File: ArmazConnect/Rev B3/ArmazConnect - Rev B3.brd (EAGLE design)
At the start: 165 x 74 mm, 59 parts, among them X0 NC3FAV2, X1 NC3FAV2, X2 NC3FAV2, X3 NC3FAV2, X4 NC5FAV-SW, X5 NC5MAV-SW, X6 NC5FAV-SW, X8 87832-26

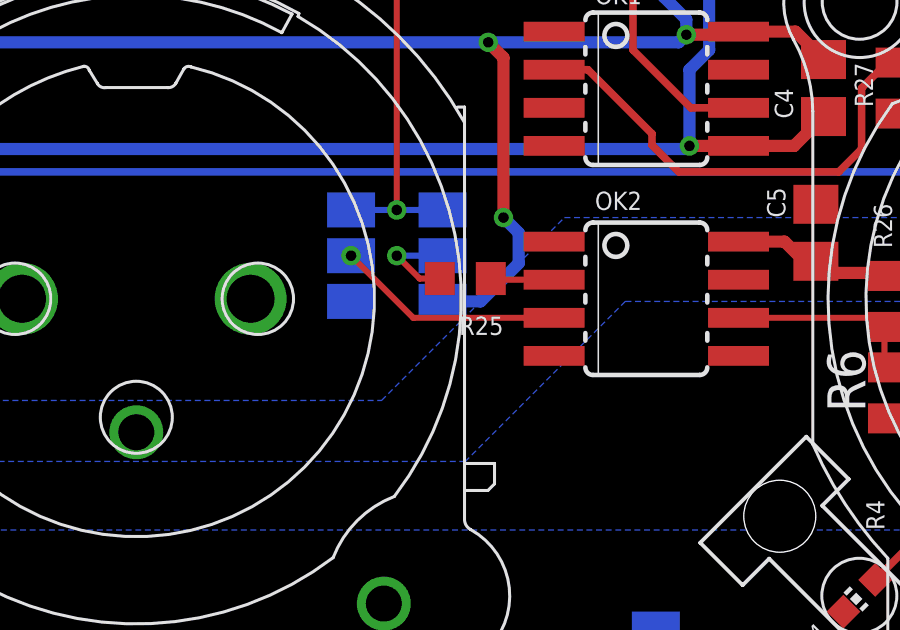
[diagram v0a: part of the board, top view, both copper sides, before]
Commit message: Revert "Update Armaz schematic and board, generate GERBER file"
This reverts commit 24852c679122bbaf0d2032972172e40d6d3f08fb.
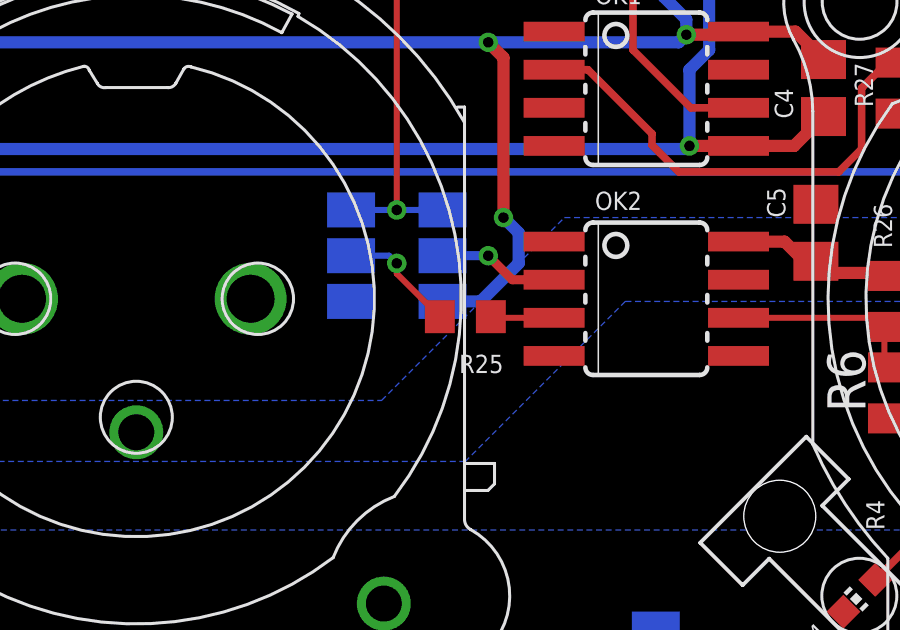
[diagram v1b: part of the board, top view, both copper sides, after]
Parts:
- moved R25 1.27 mm to (125.0, 57.4)
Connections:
- removed net N$10: OK2.2, R25.1
- removed net N$11: R25.2, SJ1.2
- new net N$17: OK2.3, R25.1
- new net UART5_TXD4: R25.2, SJ2.2
- net N$9: now also OK2.2, SJ1.2; no longer OK2.3, SJ2.2
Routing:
- net UART5_TXD4: track 0.00 -> 4.00 mm, vias 0 -> 1
- net N$9: track 7.63 -> 4.05 mm
- net N$11: track 3.28 -> 0.00 mm, vias 1 -> 0
- net N$17: track 0.00 -> 2.12 mm
- net N$10: track 2.12 -> 0.00 mm
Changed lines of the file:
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@@
 <layer number="14" name="Route14" color="1" fill="6" visible="no" active="no"/>
 <layer number="15" name="Route15" color="19" fill="6" visible="no" active="no"/>
-<layer number="16" name="Bottom" color="21" fill="1" visible="no" active="yes"/>
+<layer number="16" name="Bottom" color="21" fill="1" visible="yes" active="yes"/>
 <layer number="17" name="Pads" color="18" fill="1" visible="yes" active="yes"/>
 <layer number="18" name="Vias" color="38" fill="1" visible="yes" active="yes"/>
@@
 <layer number="20" name="Dimension" color="7" fill="1" visible="yes" active="yes"/>
 <layer number="21" name="tPlace" color="55" fill="1" visible="yes" active="yes"/>
-<layer number="22" name="bPlace" color="54" fill="1" visible="no" active="yes"/>
+<layer number="22" name="bPlace" color="54" fill="1" visible="yes" active="yes"/>
 <layer number="23" name="tOrigins" color="15" fill="1" visible="yes" active="yes"/>
-<layer number="24" name="bOrigins" color="15" fill="1" visible="no" active="yes"/>
-<layer number="25" name="tNames" color="55" fill="1" visible="yes" active="yes"/>
+<layer number="24" name="bOrigins" color="15" fill="1" visible="yes" active="yes"/>
+<layer number="25" name="tNames" color="55" fill="1" visible="no" active="yes"/>
 <layer number="26" name="bNames" color="54" fill="1" visible="no" active="yes"/>
-<layer number="27" name="tValues" color="53" fill="1" visible="yes" active="yes"/>
+<layer number="27" name="tValues" color="53" fill="1" visible="no" active="yes"/>
 <layer number="28" name="bValues" color="52" fill="1" visible="no" active="yes"/>
 <layer number="29" name="tStop" color="7" fill="3" visible="no" active="yes"/>
@@
 <layer number="49" name="Reference" color="48" fill="1" visible="yes" active="yes"/>
 <layer number="50" name="dxf" color="7" fill="1" visible="no" active="no"/>
-<layer number="51" name="tDocu" color="55" fill="1" visible="yes" active="yes"/>
+<layer number="51" name="tDocu" color="55" fill="1" visible="no" active="yes"/>
 <layer number="52" name="bDocu" color="54" fill="1" visible="no" active="yes"/>
 <layer number="53" name="tGND_GNDA" color="7" fill="1" visible="no" active="no"/>
@@
 <attribute name="VALUE" x="131.191" y="70.739" size="0.4064" layer="27" ratio="10" rot="R270"/>
 </element>
-<element name="R25" library="rcl" package="R0603" value="100" x="124.968" y="58.674" smashed="yes" rot="R180">
-<attribute name="MF" value="MULTICOMP" x="124.968" y="58.674" size="1.778" layer="27" rot="R180" display="off"/>
-<attribute name="MPN" value="MCMR06X3300FTL" x="124.968" y="58.674" size="1.778" layer="27" rot="R180" display="off"/>
-<attribute name="OC_FARNELL" value="2073472" x="124.968" y="58.674" size="1.778" layer="27" rot="R180" display="off"/>
-<attribute name="NAME" x="126.238" y="57.404" size="0.6096" layer="25" ratio="10" rot="R180"/>
-<attribute name="VALUE" x="125.603" y="60.579" size="0.4064" layer="27" ratio="10" rot="R180"/>
+<element name="R25" library="rcl" package="R0603" value="100" x="124.968" y="57.404" smashed="yes" rot="R180">
+<attribute name="MF" value="MULTICOMP" x="124.968" y="57.404" size="1.778" layer="27" rot="R180" display="off"/>
+<attribute name="MPN" value="MCMR06X3300FTL" x="124.968" y="57.404" size="1.778" layer="27" rot="R180" display="off"/>
+<attribute name="OC_FARNELL" value="2073472" x="124.968" y="57.404" size="1.778" layer="27" rot="R180" display="off"/>
+<attribute name="NAME" x="126.238" y="56.134" size="0.6096" layer="25" ratio="10" rot="R180"/>
+<attribute name="VALUE" x="125.603" y="59.309" size="0.4064" layer="27" ratio="10" rot="R180"/>
 </element>
 <element name="R26" library="rcl" package="R0603" value="4K7, DNI" x="138.938" y="57.912" smashed="yes" rot="R90">
@@
 <wire x1="122.682" y1="60.96" x2="121.158" y2="60.96" width="0.2032" layer="16"/>
 </signal>
+<signal name="N$17">
+<contactref element="R25" pad="1"/>
+<contactref element="OK2" pad="3"/>
+<wire x1="125.818" y1="57.404" x2="125.857" y2="57.365" width="0.2032" layer="1"/>
+<wire x1="125.857" y1="57.365" x2="127.9266" y2="57.365" width="0.2032" layer="1"/>
+</signal>
 <signal name="ESW3-RX">
 <contactref element="R27" pad="1"/>
@@
 <wire x1="138.176" y1="65.024" x2="139.026" y2="65.874" width="0.254" layer="1"/>
 <wire x1="139.026" y1="65.874" x2="139.192" y2="65.874" width="0.2032" layer="1"/>
+</signal>
+<signal name="N$9">
+<contactref element="OK2" pad="2"/>
+<contactref element="SJ1" pad="2"/>
+<wire x1="124.206" y1="59.436" x2="125.73" y2="59.436" width="0.3048" layer="16"/>
+<via x="125.73" y="59.436" extent="1-16" drill="0.35"/>
+<wire x1="125.73" y1="59.436" x2="126.531" y2="58.635" width="0.3048" layer="1"/>
+<wire x1="126.531" y1="58.635" x2="127.9266" y2="58.635" width="0.3048" layer="1"/>
 </signal>
 <signal name="VDD33A1" class="1">
@@
 <via x="131.572" y="69.596" extent="1-16" drill="0.35"/>
 </signal>
-<signal name="N$9">
-<contactref element="OK2" pad="3"/>
+<signal name="UART5_TXD4">
+<contactref element="R25" pad="2"/>
 <contactref element="SJ2" pad="2"/>
-<wire x1="127.9266" y1="57.365" x2="123.229" y2="57.365" width="0.2032" layer="1"/>
-<wire x1="123.229" y1="57.365" x2="121.158" y2="59.436" width="0.2032" layer="1"/>
-<via x="121.158" y="59.436" extent="1-16" drill="0.35"/>
-</signal>
-<signal name="N$10">
-<contactref element="OK2" pad="2"/>
-<contactref element="R25" pad="1"/>
-<wire x1="127.9266" y1="58.635" x2="125.857" y2="58.635" width="0.2032" layer="1"/>
-<wire x1="125.857" y1="58.635" x2="125.818" y2="58.674" width="0.2032" layer="1"/>
-</signal>
-<signal name="N$11">
-<contactref element="R25" pad="2"/>
-<contactref element="SJ1" pad="2"/>
-<wire x1="124.118" y1="58.674" x2="123.444" y2="58.674" width="0.2032" layer="1"/>
-<wire x1="123.444" y1="58.674" x2="122.682" y2="59.436" width="0.2032" layer="1"/>
-<via x="122.682" y="59.436" extent="1-16" drill="0.35"/>
-<wire x1="122.682" y1="59.436" x2="124.206" y2="59.436" width="0.2032" layer="16"/>
+<wire x1="124.118" y1="57.404" x2="122.682" y2="58.84" width="0.2032" layer="1"/>
+<wire x1="122.682" y1="58.84" x2="122.682" y2="59.182" width="0.2032" layer="1"/>
+<via x="122.682" y="59.182" extent="1-16" drill="0.35"/>
+<wire x1="122.682" y1="59.182" x2="122.428" y2="59.436" width="0.2032" layer="16"/>
+<wire x1="122.428" y1="59.436" x2="121.158" y2="59.436" width="0.2032" layer="16"/>
 </signal>
 </signals>

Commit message: Update Armaz schematic and board, generate GERBER file
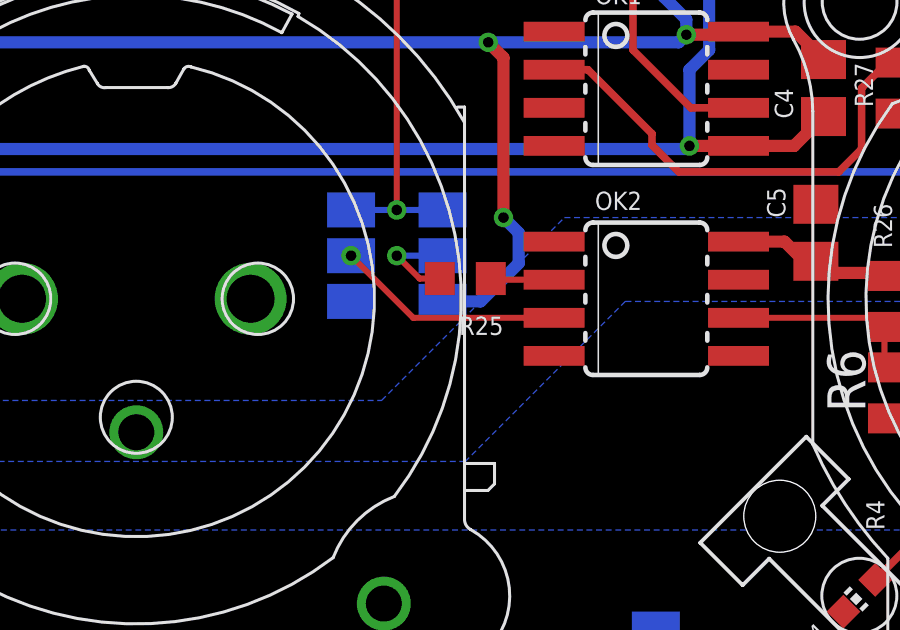
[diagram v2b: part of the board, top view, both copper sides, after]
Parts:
- moved R25 1.27 mm to (125.0, 58.7)
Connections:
- removed net N$17: OK2.3, R25.1
- removed net UART5_TXD4: R25.2, SJ2.2
- new net N$10: OK2.2, R25.1
- new net N$11: R25.2, SJ1.2
- net N$9: now also OK2.3, SJ2.2; no longer OK2.2, SJ1.2
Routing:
- net UART5_TXD4: track 4.00 -> 0.00 mm, vias 1 -> 0
- net N$9: track 4.05 -> 7.63 mm
- net N$11: track 0.00 -> 3.28 mm, vias 0 -> 1
- net N$17: track 2.12 -> 0.00 mm
- net N$10: track 0.00 -> 2.12 mm
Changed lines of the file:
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@@
 <layer number="14" name="Route14" color="1" fill="6" visible="no" active="no"/>
 <layer number="15" name="Route15" color="19" fill="6" visible="no" active="no"/>
-<layer number="16" name="Bottom" color="21" fill="1" visible="yes" active="yes"/>
+<layer number="16" name="Bottom" color="21" fill="1" visible="no" active="yes"/>
 <layer number="17" name="Pads" color="18" fill="1" visible="yes" active="yes"/>
 <layer number="18" name="Vias" color="38" fill="1" visible="yes" active="yes"/>
@@
 <layer number="20" name="Dimension" color="7" fill="1" visible="yes" active="yes"/>
 <layer number="21" name="tPlace" color="55" fill="1" visible="yes" active="yes"/>
-<layer number="22" name="bPlace" color="54" fill="1" visible="yes" active="yes"/>
+<layer number="22" name="bPlace" color="54" fill="1" visible="no" active="yes"/>
 <layer number="23" name="tOrigins" color="15" fill="1" visible="yes" active="yes"/>
-<layer number="24" name="bOrigins" color="15" fill="1" visible="yes" active="yes"/>
-<layer number="25" name="tNames" color="55" fill="1" visible="no" active="yes"/>
+<layer number="24" name="bOrigins" color="15" fill="1" visible="no" active="yes"/>
+<layer number="25" name="tNames" color="55" fill="1" visible="yes" active="yes"/>
 <layer number="26" name="bNames" color="54" fill="1" visible="no" active="yes"/>
-<layer number="27" name="tValues" color="53" fill="1" visible="no" active="yes"/>
+<layer number="27" name="tValues" color="53" fill="1" visible="yes" active="yes"/>
 <layer number="28" name="bValues" color="52" fill="1" visible="no" active="yes"/>
 <layer number="29" name="tStop" color="7" fill="3" visible="no" active="yes"/>
@@
 <layer number="49" name="Reference" color="48" fill="1" visible="yes" active="yes"/>
 <layer number="50" name="dxf" color="7" fill="1" visible="no" active="no"/>
-<layer number="51" name="tDocu" color="55" fill="1" visible="no" active="yes"/>
+<layer number="51" name="tDocu" color="55" fill="1" visible="yes" active="yes"/>
 <layer number="52" name="bDocu" color="54" fill="1" visible="no" active="yes"/>
 <layer number="53" name="tGND_GNDA" color="7" fill="1" visible="no" active="no"/>
@@
 <attribute name="VALUE" x="131.191" y="70.739" size="0.4064" layer="27" ratio="10" rot="R270"/>
 </element>
-<element name="R25" library="rcl" package="R0603" value="100" x="124.968" y="57.404" smashed="yes" rot="R180">
-<attribute name="MF" value="MULTICOMP" x="124.968" y="57.404" size="1.778" layer="27" rot="R180" display="off"/>
-<attribute name="MPN" value="MCMR06X3300FTL" x="124.968" y="57.404" size="1.778" layer="27" rot="R180" display="off"/>
-<attribute name="OC_FARNELL" value="2073472" x="124.968" y="57.404" size="1.778" layer="27" rot="R180" display="off"/>
-<attribute name="NAME" x="126.238" y="56.134" size="0.6096" layer="25" ratio="10" rot="R180"/>
-<attribute name="VALUE" x="125.603" y="59.309" size="0.4064" layer="27" ratio="10" rot="R180"/>
+<element name="R25" library="rcl" package="R0603" value="100" x="124.968" y="58.674" smashed="yes" rot="R180">
+<attribute name="MF" value="MULTICOMP" x="124.968" y="58.674" size="1.778" layer="27" rot="R180" display="off"/>
+<attribute name="MPN" value="MCMR06X3300FTL" x="124.968" y="58.674" size="1.778" layer="27" rot="R180" display="off"/>
+<attribute name="OC_FARNELL" value="2073472" x="124.968" y="58.674" size="1.778" layer="27" rot="R180" display="off"/>
+<attribute name="NAME" x="126.238" y="57.404" size="0.6096" layer="25" ratio="10" rot="R180"/>
+<attribute name="VALUE" x="125.603" y="60.579" size="0.4064" layer="27" ratio="10" rot="R180"/>
 </element>
 <element name="R26" library="rcl" package="R0603" value="4K7, DNI" x="138.938" y="57.912" smashed="yes" rot="R90">
@@
 <wire x1="122.682" y1="60.96" x2="121.158" y2="60.96" width="0.2032" layer="16"/>
 </signal>
-<signal name="N$17">
-<contactref element="R25" pad="1"/>
-<contactref element="OK2" pad="3"/>
-<wire x1="125.818" y1="57.404" x2="125.857" y2="57.365" width="0.2032" layer="1"/>
-<wire x1="125.857" y1="57.365" x2="127.9266" y2="57.365" width="0.2032" layer="1"/>
-</signal>
 <signal name="ESW3-RX">
 <contactref element="R27" pad="1"/>
@@
 <wire x1="138.176" y1="65.024" x2="139.026" y2="65.874" width="0.254" layer="1"/>
 <wire x1="139.026" y1="65.874" x2="139.192" y2="65.874" width="0.2032" layer="1"/>
-</signal>
-<signal name="N$9">
-<contactref element="OK2" pad="2"/>
-<contactref element="SJ1" pad="2"/>
-<wire x1="124.206" y1="59.436" x2="125.73" y2="59.436" width="0.3048" layer="16"/>
-<via x="125.73" y="59.436" extent="1-16" drill="0.35"/>
-<wire x1="125.73" y1="59.436" x2="126.531" y2="58.635" width="0.3048" layer="1"/>
-<wire x1="126.531" y1="58.635" x2="127.9266" y2="58.635" width="0.3048" layer="1"/>
 </signal>
 <signal name="VDD33A1" class="1">
@@
 <via x="131.572" y="69.596" extent="1-16" drill="0.35"/>
 </signal>
-<signal name="UART5_TXD4">
+<signal name="N$9">
+<contactref element="OK2" pad="3"/>
+<contactref element="SJ2" pad="2"/>
+<wire x1="127.9266" y1="57.365" x2="123.229" y2="57.365" width="0.2032" layer="1"/>
+<wire x1="123.229" y1="57.365" x2="121.158" y2="59.436" width="0.2032" layer="1"/>
+<via x="121.158" y="59.436" extent="1-16" drill="0.35"/>
+</signal>
+<signal name="N$10">
+<contactref element="OK2" pad="2"/>
+<contactref element="R25" pad="1"/>
+<wire x1="127.9266" y1="58.635" x2="125.857" y2="58.635" width="0.2032" layer="1"/>
+<wire x1="125.857" y1="58.635" x2="125.818" y2="58.674" width="0.2032" layer="1"/>
+</signal>
+<signal name="N$11">
 <contactref element="R25" pad="2"/>
-<contactref element="SJ2" pad="2"/>
-<wire x1="124.118" y1="57.404" x2="122.682" y2="58.84" width="0.2032" layer="1"/>
-<wire x1="122.682" y1="58.84" x2="122.682" y2="59.182" width="0.2032" layer="1"/>
-<via x="122.682" y="59.182" extent="1-16" drill="0.35"/>
-<wire x1="122.682" y1="59.182" x2="122.428" y2="59.436" width="0.2032" layer="16"/>
-<wire x1="122.428" y1="59.436" x2="121.158" y2="59.436" width="0.2032" layer="16"/>
+<contactref element="SJ1" pad="2"/>
+<wire x1="124.118" y1="58.674" x2="123.444" y2="58.674" width="0.2032" layer="1"/>
+<wire x1="123.444" y1="58.674" x2="122.682" y2="59.436" width="0.2032" layer="1"/>
+<via x="122.682" y="59.436" extent="1-16" drill="0.35"/>
+<wire x1="122.682" y1="59.436" x2="124.206" y2="59.436" width="0.2032" layer="16"/>
 </signal>
 </signals>
